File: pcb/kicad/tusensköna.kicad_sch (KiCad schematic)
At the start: 36 parts, among them J1 AudioJack3, J2 AudioJack3, J3 Micro_SD_Card, SW1 SW_Push, SW2 SW_Push, U1 Electrosmith_Daisy_Seed_Rev4

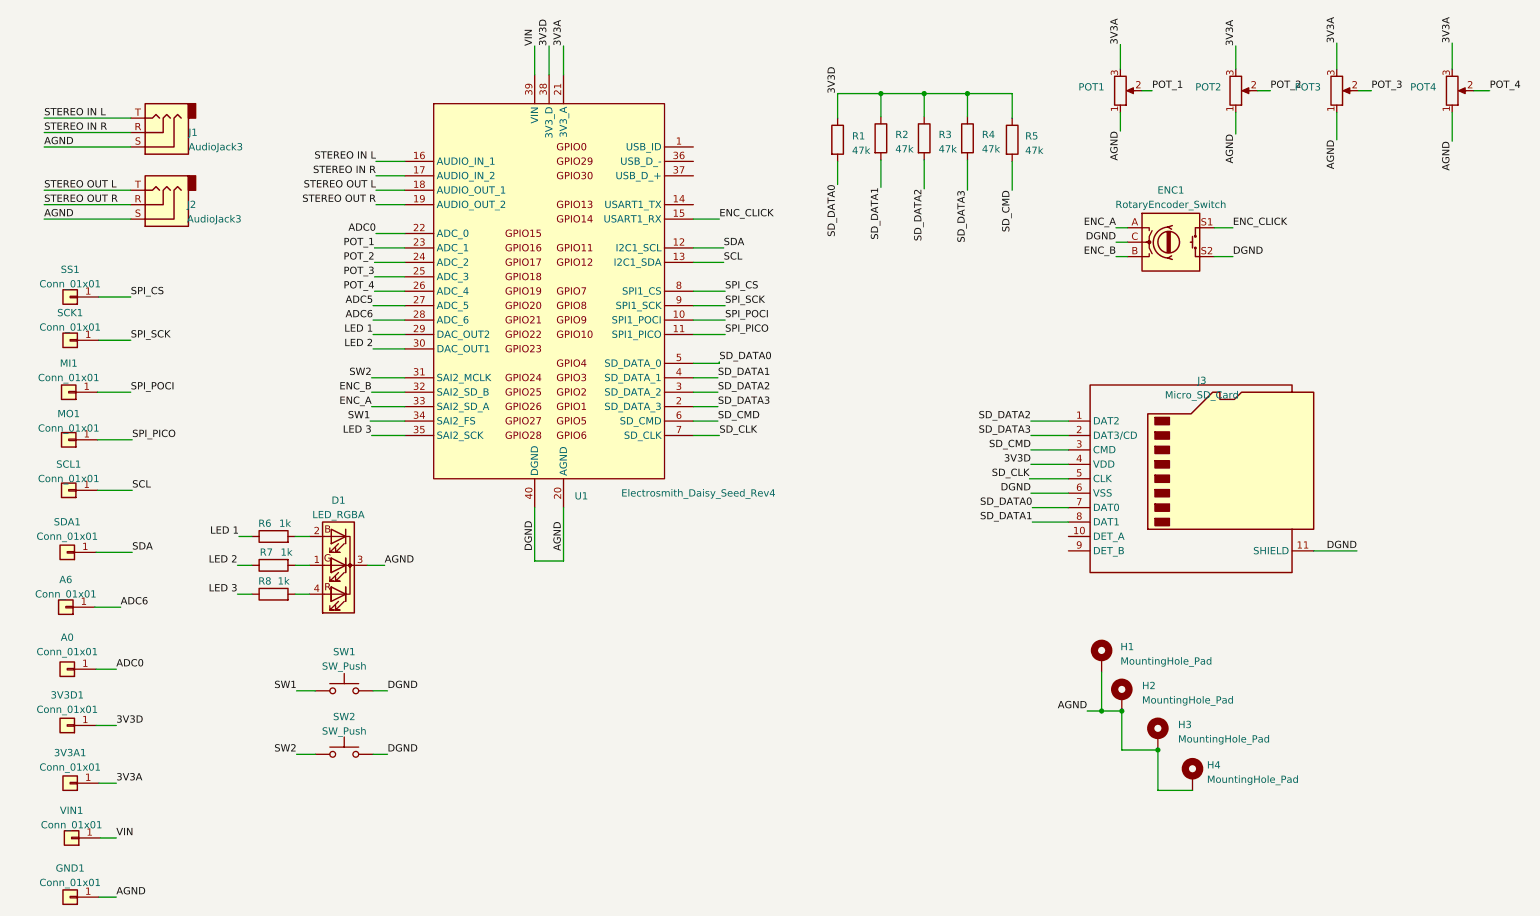
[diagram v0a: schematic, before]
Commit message: issues fixed
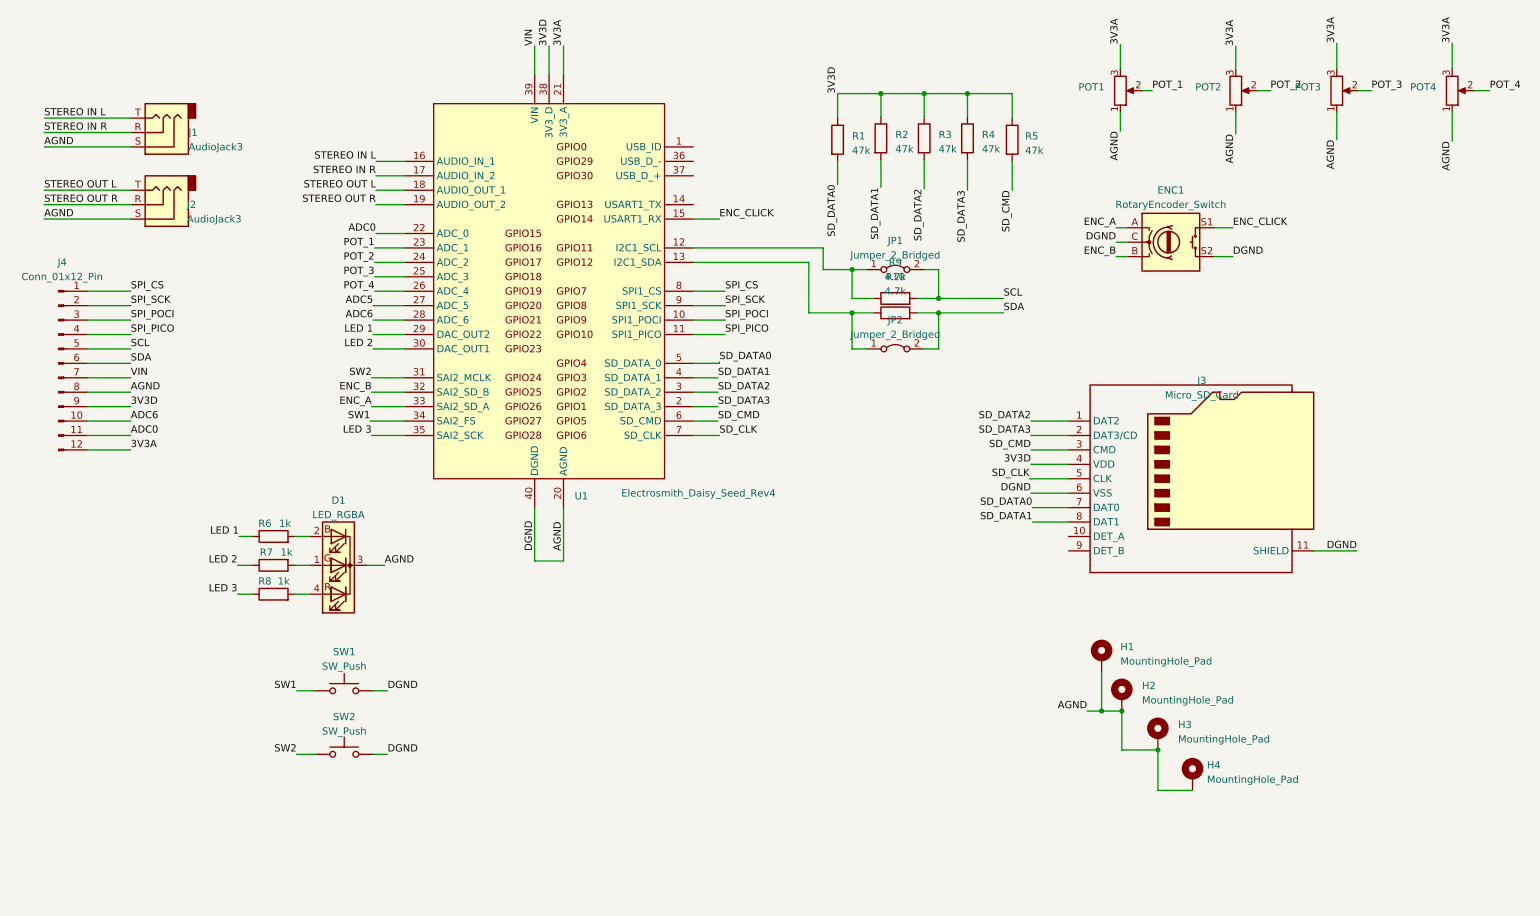
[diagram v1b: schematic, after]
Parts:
- removed 3V3A1, 3V3D1, A0, A6, GND1, MI1, MO1, SCK1, SCL1, SDA1, SS1, VIN1: Conn_01x01, Connector_Wire:SolderWire-0.5sqmm_1x01_D0.9mm_OD2.1mm, symbol Connector_Generic:Conn_01x01
- added J4: Conn_01x12_Pin, Connector_PinHeader_2.54mm:PinHeader_1x12_P2.54mm_Vertical, symbol Connector:Conn_01x12_Pin
- added JP1, JP2: Jumper_2_Bridged, Connector_PinHeader_2.54mm:PinHeader_1x02_P2.54mm_Vertical, symbol Jumper:Jumper_2_Bridged
- added R10, R9: 4.7k, Resistor_SMD:R_0805_2012Metric, symbol Device:R
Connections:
- net 3V3A: now also J4.12 (Pin_12)
- net 3V3D: now also J4.9 (Pin_9)
- net ADC0: now also J4.11 (Pin_11)
- net ADC6: now also J4.10 (Pin_10)
- net AGND: now also J4.8 (Pin_8)
- net SCL: now also J4.5 (Pin_5), JP1.2 (B), R9.2; no longer U1.13 (I2C1_SDA)
- net SDA: now also J4.6 (Pin_6), JP2.2 (B), R10.2; no longer U1.12 (I2C1_SCL)
- net SPI_CS: now also J4.1 (Pin_1)
- net SPI_PICO: now also J4.4 (Pin_4)
- net SPI_POCI: now also J4.3 (Pin_3)
- net SPI_SCK: now also J4.2 (Pin_2)
- net VIN: now also J4.7 (Pin_7)
- new net: JP1.1 (A), R9.1, U1.12 (I2C1_SCL)
- new net: JP2.1 (A), R10.1, U1.13 (I2C1_SDA)

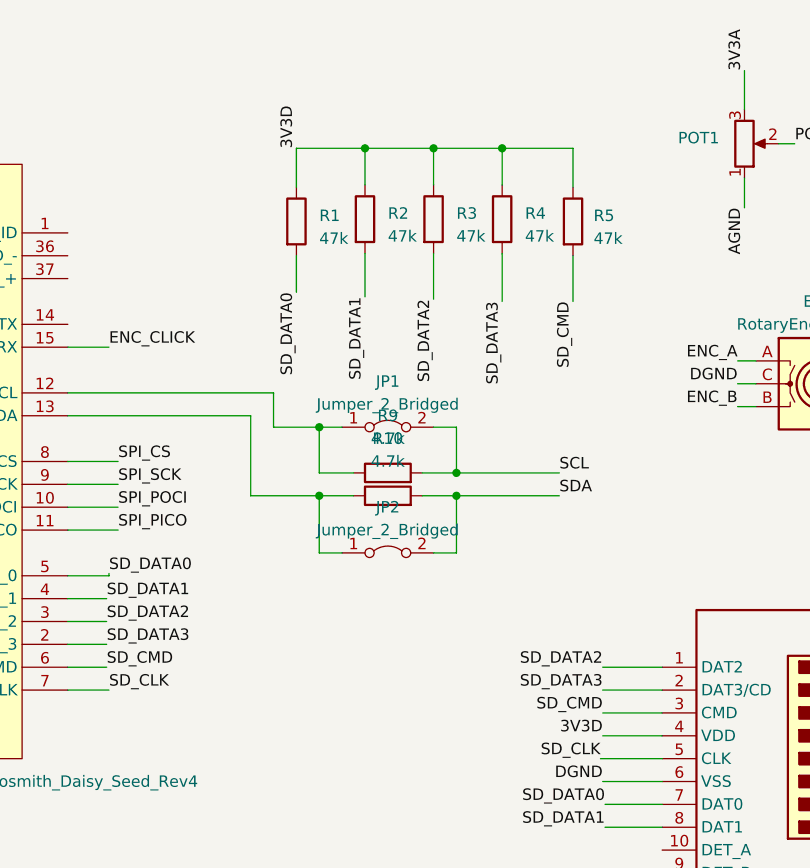
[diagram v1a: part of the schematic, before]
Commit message: pullup
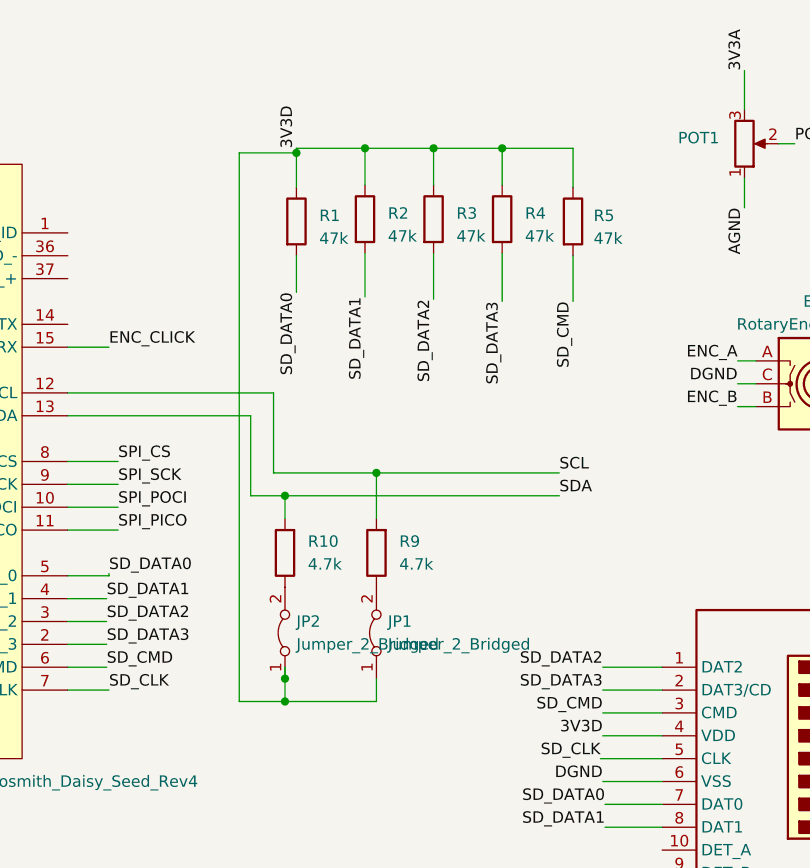
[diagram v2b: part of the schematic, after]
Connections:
- net 3V3D: now also JP1.1 (A), JP2.1 (A)
- net SCL: now also U1.12 (I2C1_SCL); no longer JP1.2 (B)
- net SDA: now also U1.13 (I2C1_SDA); no longer JP2.2 (B)
- new net: JP1.2 (B), R9.1
- new net: JP2.2 (B), R10.1
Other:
- moved on the sheet: JP1, JP2, R10, R9
